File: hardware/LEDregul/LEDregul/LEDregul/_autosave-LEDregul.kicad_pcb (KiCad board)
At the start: 2 copper layers, 97.8 x 67.3 mm, 45 parts, among them J1 Conn_02x04_Odd_Even, J2 Conn_01x04_Male, J4 Conn_01x20_Female, U1 FAN5341, U2 FAN5341, U3 FAN5341, U4 FAN5341, X1 SiT1534

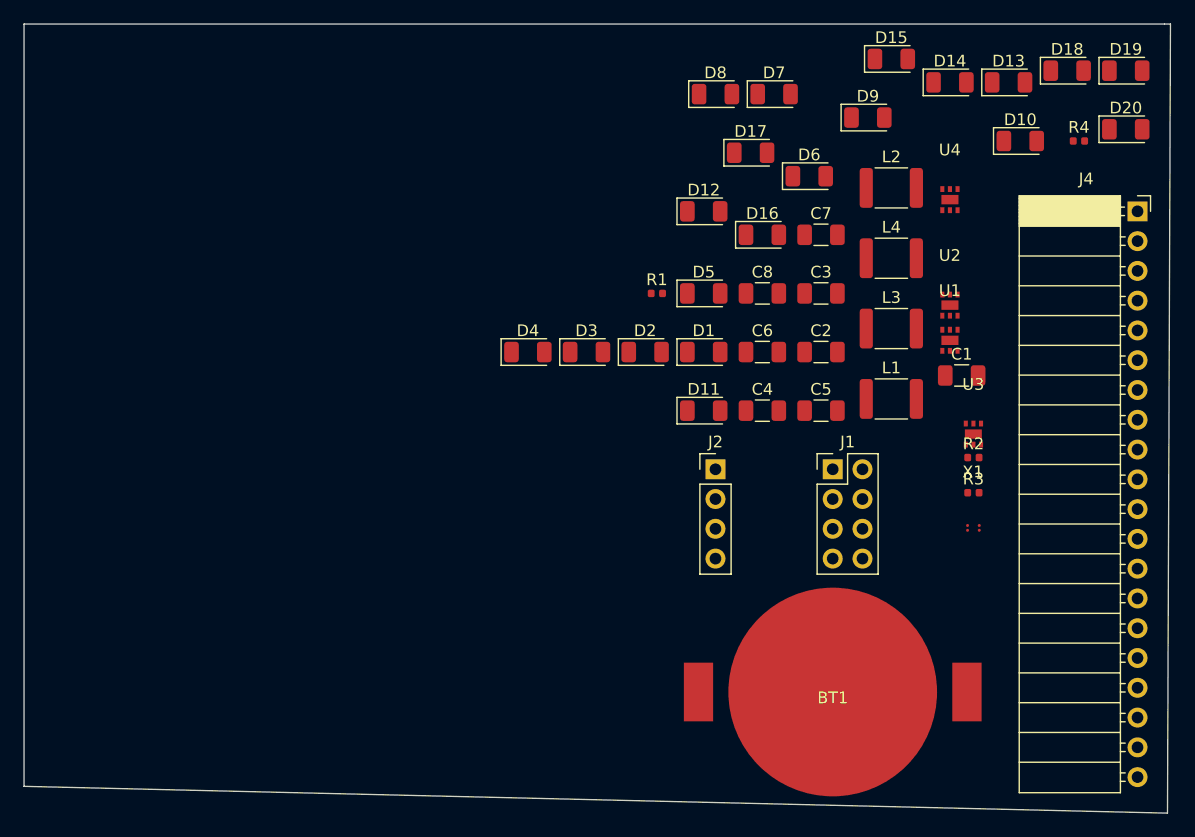
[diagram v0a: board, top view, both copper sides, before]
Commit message: nRF52 start
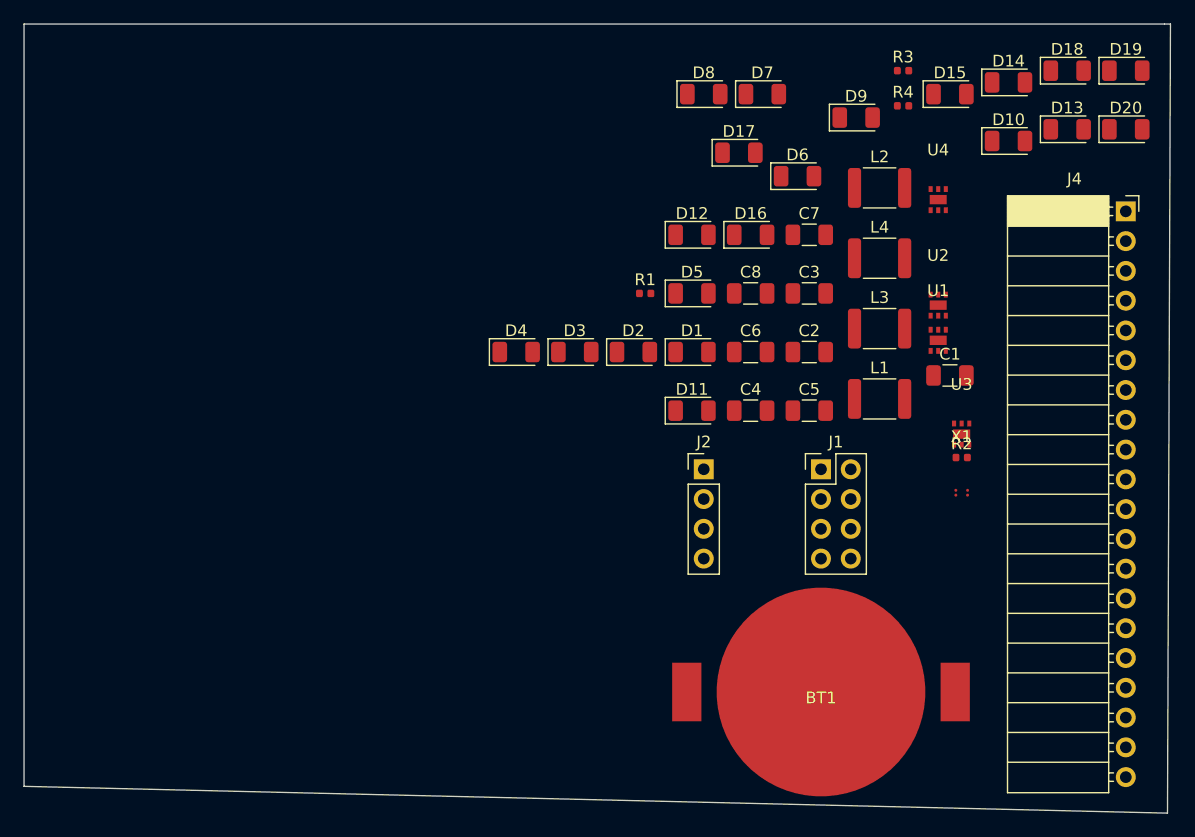
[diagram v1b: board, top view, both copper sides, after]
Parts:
- moved R3 36.5 mm to (108.0, 53.0)
- moved R4 15.3 mm to (108.0, 56.0)
- moved D13 6.40 mm to (122.0, 58.0)
- moved D15 5.83 mm to (112.0, 55.0)
- moved D14 5.00 mm to (117.0, 54.0)
- moved X1 3.16 mm to (113.0, 89.0)
- moved D12 2.24 mm to (90.0, 67.0)
- moved BT1 1.00 mm to (101.0, 106.0)
- moved C1 1.00 mm to (112.0, 79.0)
- moved C2 1.00 mm to (100.0, 77.0)
- moved C3 1.00 mm to (100.0, 72.0)
- moved C4 1.00 mm to (95.0, 82.0)
- moved C5 1.00 mm to (100.0, 82.0)
- moved C6 1.00 mm to (95.0, 77.0)
- moved C7 1.00 mm to (100.0, 67.0)
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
